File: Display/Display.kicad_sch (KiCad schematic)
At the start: 9 parts, among them J1 Conn_01x60, J2 12402032E202A, J3 12402032E202A, J4 Conn_01x60

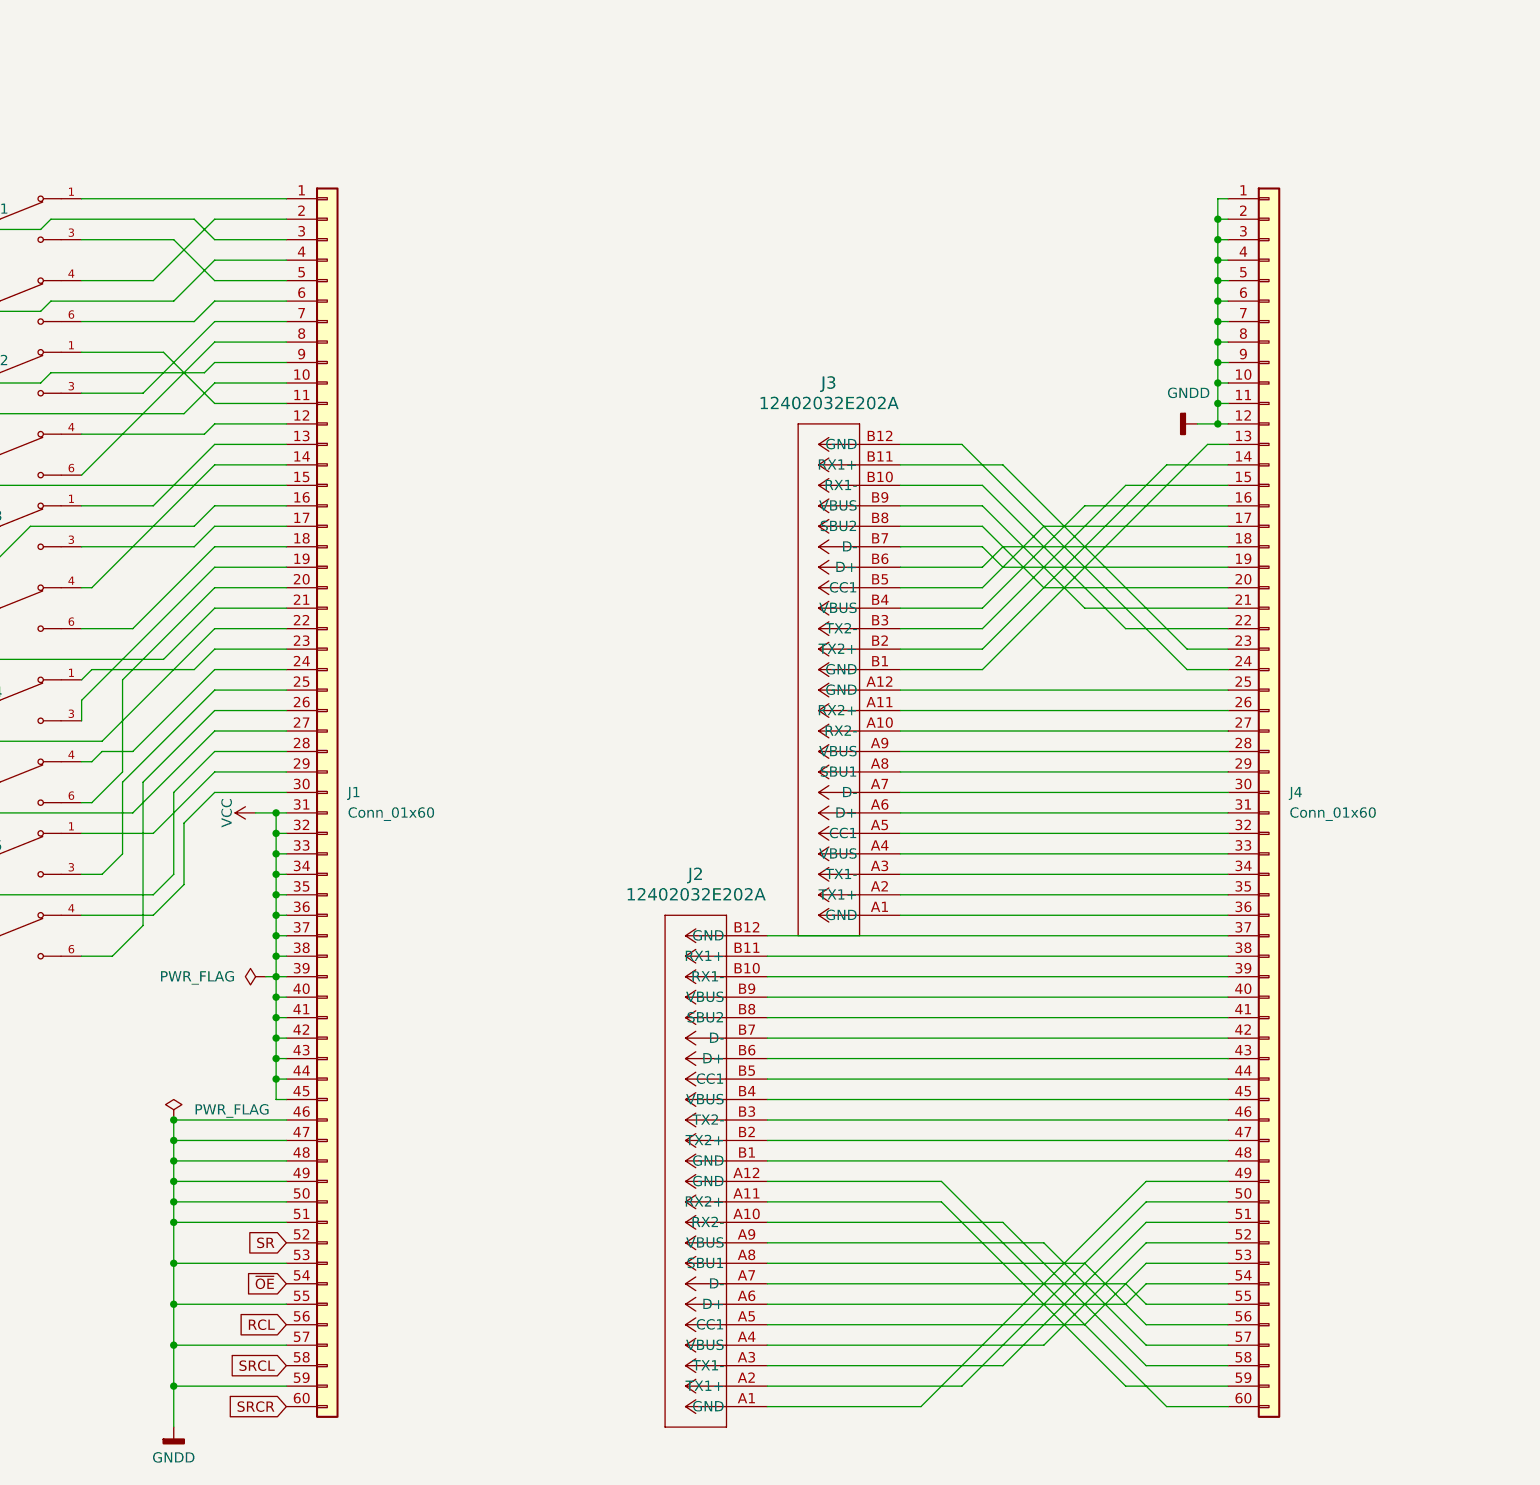
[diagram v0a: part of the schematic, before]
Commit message: quick save
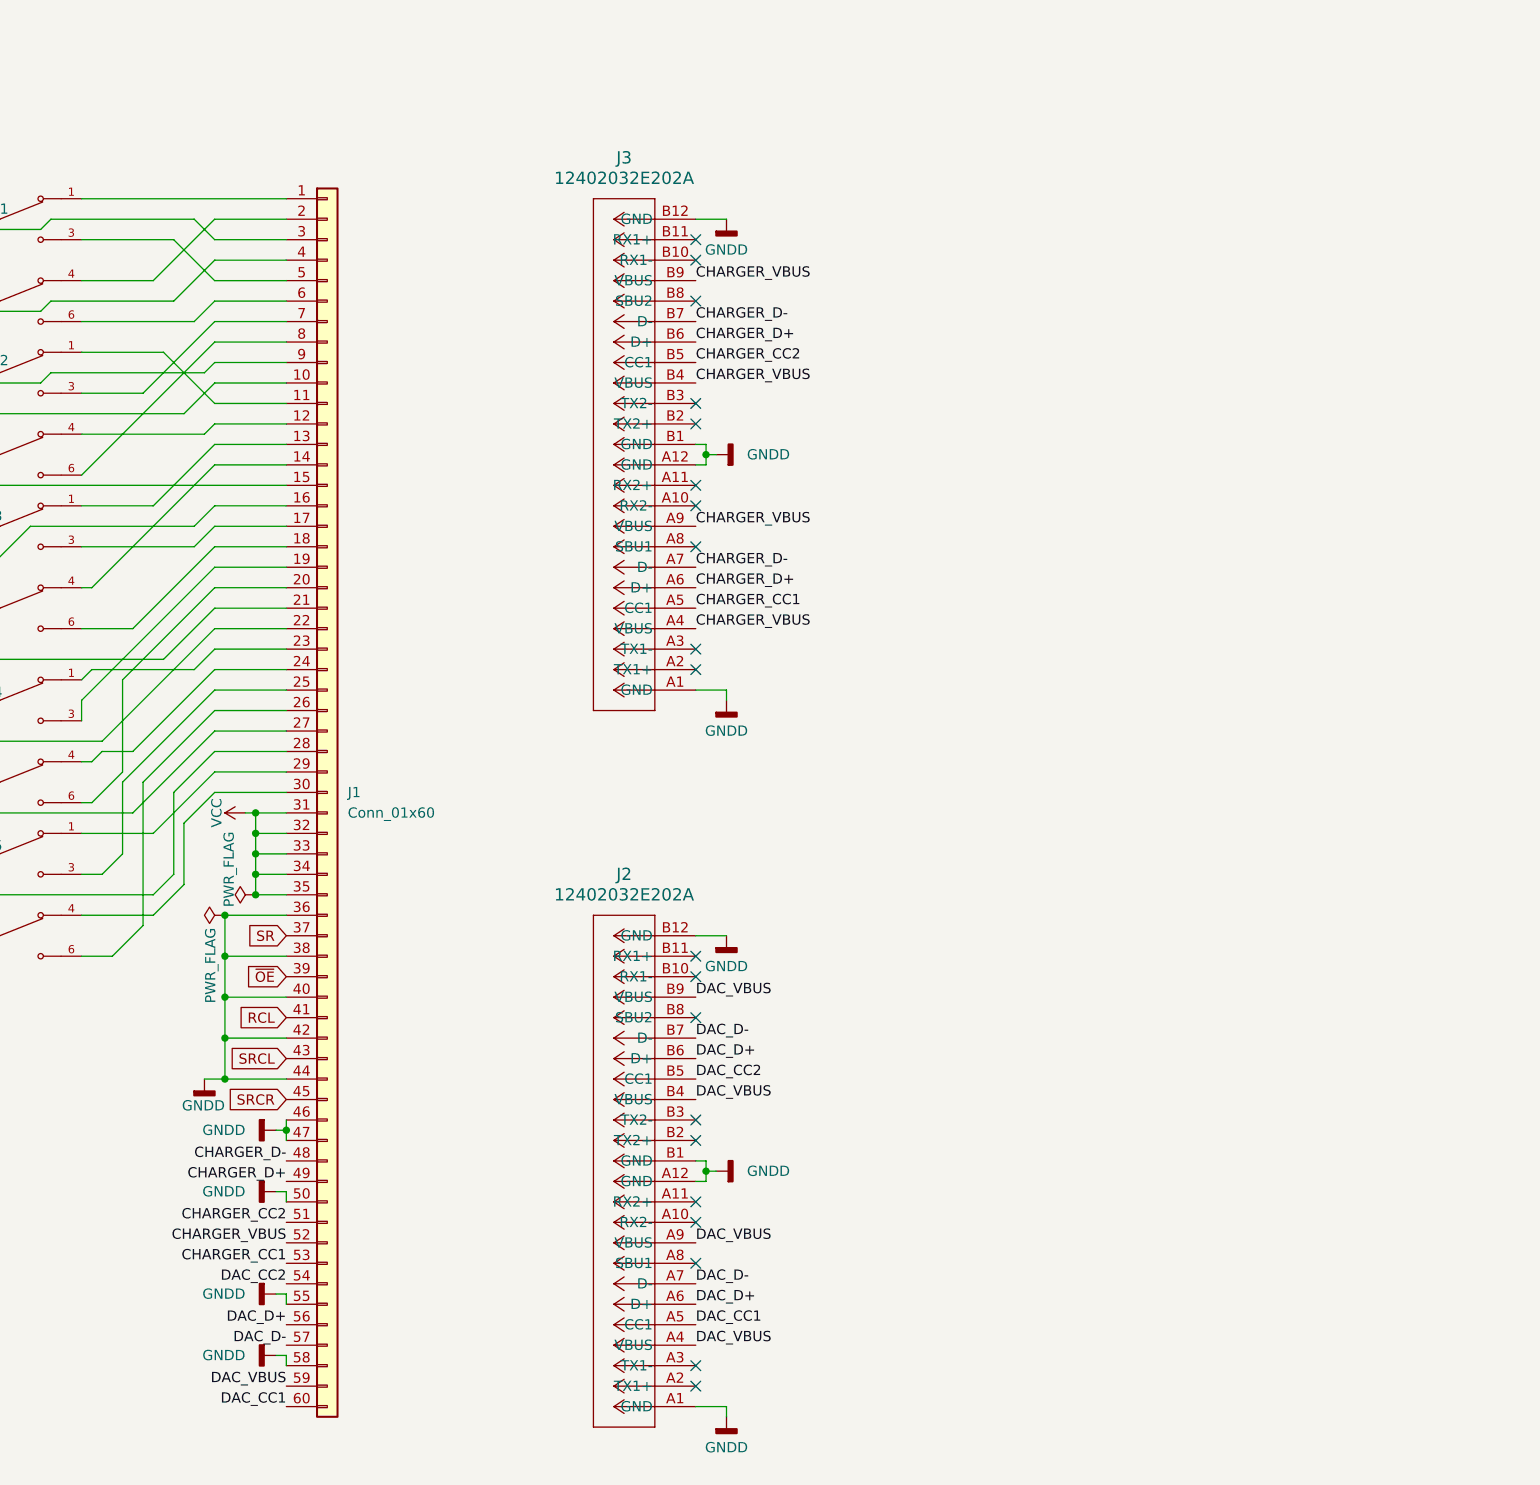
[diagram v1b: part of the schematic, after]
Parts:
- removed J4: Conn_01x60, External_Parts:CON_2004850460_MOL, symbol Connector_Generic:Conn_01x60
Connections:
- net GNDD: now also J1.36 (Pin_36), J1.38 (Pin_38), J1.40 (Pin_40), J1.42 (Pin_42), J1.44 (Pin_44), J1.58 (Pin_58), J2.A1 (GND), J2.A12 (GND), J2.B1 (GND), J2.B12 (GND), J3.A1 (GND), J3.A12 (GND), J3.B1 (GND), J3.B12 (GND); no longer J1.48 (Pin_48), J1.49 (Pin_49), J1.51 (Pin_51), J1.53 (Pin_53), J1.57 (Pin_57), J1.59 (Pin_59)
- net RCL: now also J1.41 (Pin_41); no longer J1.56 (Pin_56)
- net SR: now also J1.37 (Pin_37); no longer J1.52 (Pin_52)
- net SRCL: now also J1.43 (Pin_43); no longer J1.58 (Pin_58)
- net SRCR: now also J1.45 (Pin_45); no longer J1.60 (Pin_60)
- net VCC: no longer J1.36 (Pin_36), J1.37 (Pin_37), J1.38 (Pin_38), J1.39 (Pin_39), J1.40 (Pin_40), J1.41 (Pin_41), J1.42 (Pin_42), J1.43 (Pin_43), J1.44 (Pin_44), J1.45 (Pin_45)
- net ~{OE}: now also J1.39 (Pin_39); no longer J1.54 (Pin_54)
- net CHARGER_VBUS: now reaches J3.A4 (VBUS)
- net CHARGER_VBUS: now also J1.52 (Pin_52), J3.A9 (VBUS), J3.B4 (VBUS), J3.B9 (VBUS)
- net CHARGER_CC1: now reaches J3.A5 (CC1)
- net CHARGER_CC1: now also J1.53 (Pin_53)
- net CHARGER_D+: now reaches J3.A6 (D+)
- net CHARGER_D+: now also J1.49 (Pin_49), J3.B6 (D+)
- net CHARGER_D-: now reaches J3.A7 (D-)
- net CHARGER_D-: now also J1.48 (Pin_48), J3.B7 (D-)
- net CHARGER_CC2: now reaches J3.B5 (CC1)
- net CHARGER_CC2: now also J1.51 (Pin_51)
- net DAC_VBUS: now reaches J2.B9 (VBUS)
- net DAC_VBUS: now also J1.59 (Pin_59), J2.A4 (VBUS), J2.A9 (VBUS), J2.B4 (VBUS)
- net DAC_D-: now reaches J2.B7 (D-)
- net DAC_D-: now also J1.57 (Pin_57), J2.A7 (D-)
- net DAC_D+: now reaches J2.B6 (D+)
- net DAC_D+: now also J1.56 (Pin_56), J2.A6 (D+)
- net DAC_CC2: now reaches J2.B5 (CC1)
- net DAC_CC2: now also J1.54 (Pin_54)
- net DAC_CC1: now reaches J2.A5 (CC1)
- net DAC_CC1: now also J1.60 (Pin_60)
- no-connect marks 1 -> 21
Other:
- moved on the sheet: J2
